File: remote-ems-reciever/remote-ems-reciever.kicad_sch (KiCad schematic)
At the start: 39 parts, among them IC1 Wio-E5, IC2 MCP2562, J1 Conn_Coaxial, J2 Conn_01x04, J3 Conn_01x04, J4 Conn_01x04_Pin, J5 Conn_01x04, Q1 BSS138, SW1 SW_Push, SW2 SW_Push, SW3 SW_Push, SW4 SW_DIP_x02, U1 STM32G431K8Tx, U2 NJM12888F33

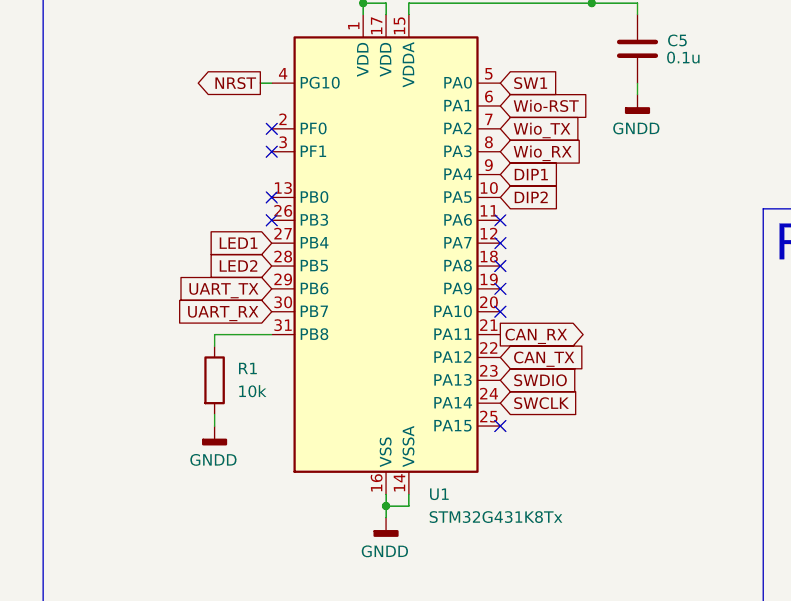
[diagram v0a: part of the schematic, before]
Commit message: remote-ems-reciever　ビア、シルク、LED以外完成
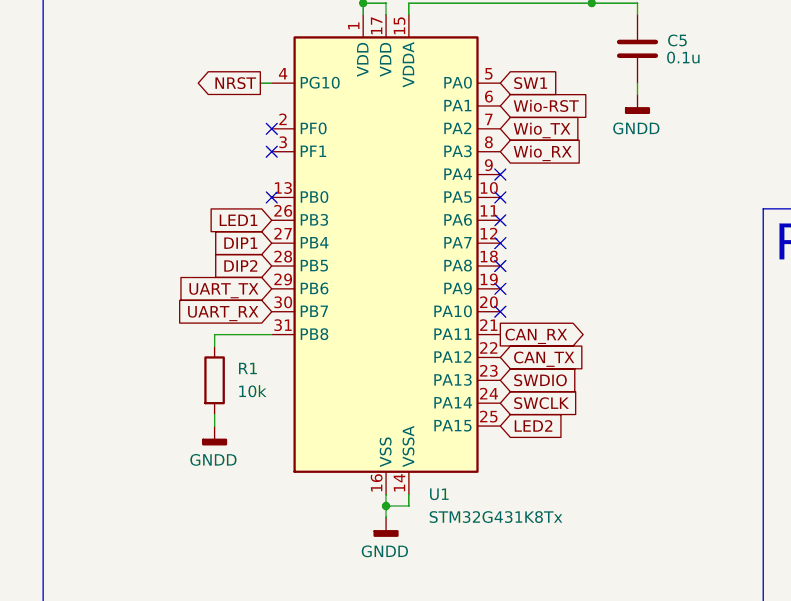
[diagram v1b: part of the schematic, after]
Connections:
- net DIP1: now also U1.27 (PB4); no longer U1.9 (PA4)
- net DIP2: now also U1.28 (PB5); no longer U1.10 (PA5)
- net LED1: now also U1.26 (PB3); no longer U1.27 (PB4)
- net LED2: now also U1.25 (PA15); no longer U1.28 (PB5)
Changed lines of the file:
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@@
+	)
+	(no_connect
+		(at 63.5 55.88)
 	)
 	(no_connect
@@
 	)
 	(no_connect
-		(at 63.5 83.82)
-	)
-	(no_connect
 		(at 38.1 50.8)
 	)
@@
 	)
 	(no_connect
-		(at 38.1 60.96)
-	)
-	(no_connect
 		(at 39.37 152.4)
 	)
@@
 	(no_connect
 		(at 69.85 149.86)
+	)
+	(no_connect
+		(at 63.5 58.42)
 	)
 	(no_connect
@@
 	(global_label "DIP1"
 		(shape input)
-		(at 63.5 55.88 0)
+		(at 38.1 63.5 180)
+		(fields_autoplaced yes)
+		(effects
+			(font
+				(size 1.27 1.27)
+			)
+			(justify right)
+		)
+		(property "Intersheetrefs" "${INTERSHEET_REFS}"
+			(at 30.7605 63.5 0)
+			(effects
+				(font
+					(size 1.27 1.27)
+				)
+				(justify right)
+				(hide yes)
+			)
+		)
+	)
+	(global_label "SWCLK"
+		(shape input)
+		(at 245.872 31.75 0)
 		(fields_autoplaced yes)
 		(effects
@@
 		)
 		(property "Intersheetrefs" "${INTERSHEET_REFS}"
-			(at 70.8395 55.88 0)
+			(at 255.0862 31.75 0)
 			(effects
 				(font
@@
 		)
 	)
-	(global_label "SWCLK"
-		(shape input)
-		(at 245.872 31.75 0)
-		(fields_autoplaced yes)
-		(effects
-			(font
-				(size 1.27 1.27)
-			)
-			(justify left)
-		)
-		(property "Intersheetrefs" "${INTERSHEET_REFS}"
-			(at 255.0862 31.75 0)
-			(effects
-				(font
-					(size 1.27 1.27)
-				)
-				(justify left)
-				(hide yes)
-			)
-		)
-	)
 	(global_label "LED2"
 		(shape input)
@@
 	(global_label "LED1"
 		(shape input)
-		(at 38.1 63.5 180)
+		(at 38.1 60.96 180)
 		(fields_autoplaced yes)
 		(effects
@@
 		)
 		(property "Intersheetrefs" "${INTERSHEET_REFS}"
-			(at 30.4582 63.5 0)
+			(at 30.4582 60.96 0)
 			(effects
 				(font
@@
 	(global_label "LED2"
 		(shape input)
+		(at 63.5 83.82 0)
+		(fields_autoplaced yes)
+		(effects
+			(font
+				(size 1.27 1.27)
+			)
+			(justify left)
+		)
+		(property "Intersheetrefs" "${INTERSHEET_REFS}"
+			(at 71.1418 83.82 0)
+			(effects
+				(font
+					(size 1.27 1.27)
+				)
+				(justify left)
+				(hide yes)
+			)
+		)
+	)
+	(global_label "LED1"
+		(shape input)
+		(at 161.29 140.97 180)
+		(fields_autoplaced yes)
+		(effects
+			(font
+				(size 1.27 1.27)
+			)
+			(justify right)
+		)
+		(property "Intersheetrefs" "${INTERSHEET_REFS}"
+			(at 153.6482 140.97 0)
+			(effects
+				(font
+					(size 1.27 1.27)
+				)
+				(justify right)
+				(hide yes)
+			)
+		)
+	)
+	(global_label "DIP2"
+		(shape input)
 		(at 38.1 66.04 180)
 		(fields_autoplaced yes)
@@
 		)
 		(property "Intersheetrefs" "${INTERSHEET_REFS}"
-			(at 30.4582 66.04 0)
+			(at 30.7605 66.04 0)
 			(effects
 				(font
@@
 				(hide yes)
 			)
-		)
-	)
-	(global_label "LED1"
-		(shape input)
-		(at 161.29 140.97 180)
-		(fields_autoplaced yes)
-		(effects
-			(font
-				(size 1.27 1.27)
-			)
-			(justify right)
-		)
-		(property "Intersheetrefs" "${INTERSHEET_REFS}"
-			(at 153.6482 140.97 0)
-			(effects
-				(font
-					(size 1.27 1.27)
-				)
-				(justify right)
-				(hide yes)
-			)
-		)
-	)
-	(global_label "DIP2"
-		(shape input)
-		(at 63.5 58.42 0)
-		(fields_autoplaced yes)
-		(effects
-			(font
-				(size 1.27 1.27)
-			)
-			(justify left)
-		)
-		(property "Intersheetrefs" "${INTERSHEET_REFS}"
-			(at 70.8395 58.42 0)
-			(effects
-				(font
-					(size 1.27 1.27)
-				)
-				(justify left)
-				(hide yes)
-			)
